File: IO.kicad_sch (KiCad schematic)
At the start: 0 parts

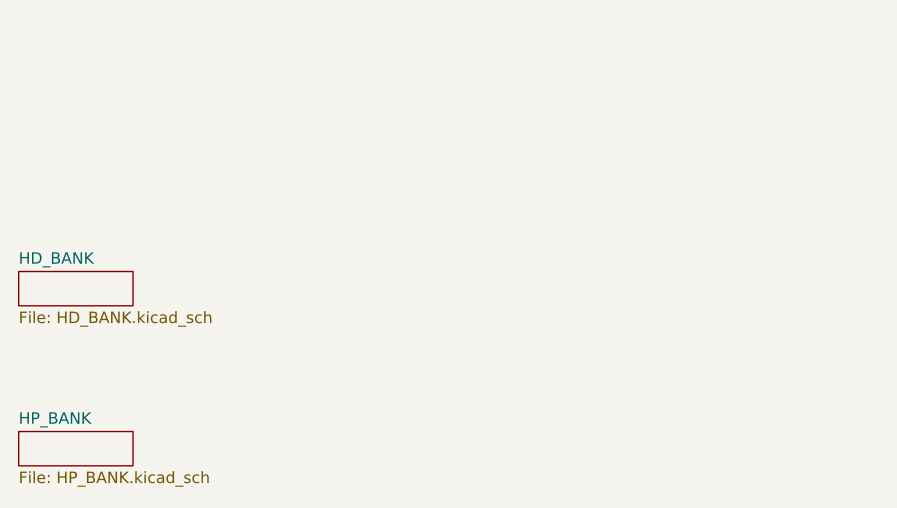
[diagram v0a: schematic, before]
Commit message: finishing schematic
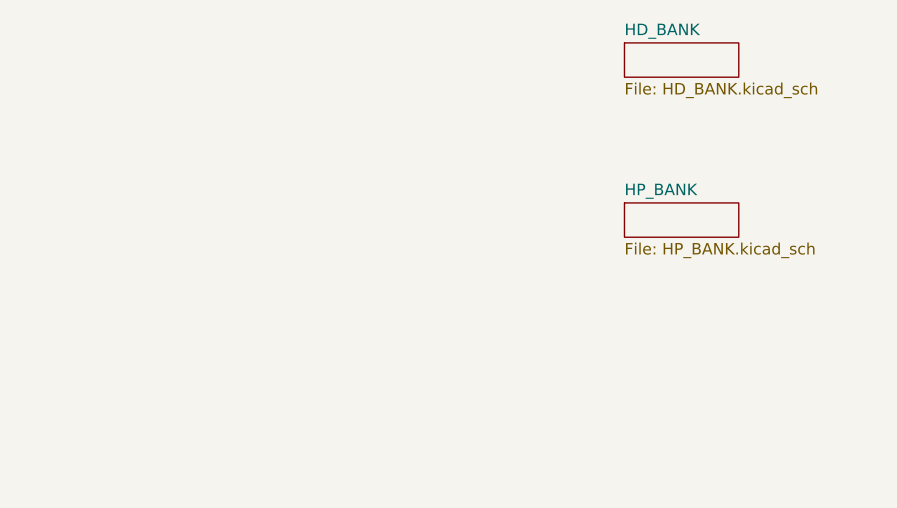
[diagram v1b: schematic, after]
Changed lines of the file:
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@@
 	(paper "A4")
 	(sheet
-		(at 74.93 121.92)
+		(at 142.24 96.52)
 		(size 12.7 3.81)
 		(exclude_from_sim no)
@@
 		)
 		(property "Sheetname" "HP_BANK"
-			(at 74.93 121.2084 0)
+			(at 142.24 95.8084 0)
 			(show_name no)
 			(do_not_autoplace no)
@@
 		)
 		(property "Sheetfile" "HP_BANK.kicad_sch"
-			(at 74.93 126.3146 0)
+			(at 142.24 100.9146 0)
 			(show_name no)
 			(do_not_autoplace no)
@@
 	)
 	(sheet
-		(at 74.93 104.14)
+		(at 142.24 78.74)
 		(size 12.7 3.81)
 		(exclude_from_sim no)
@@
 		)
 		(property "Sheetname" "HD_BANK"
-			(at 74.93 103.4284 0)
+			(at 142.24 78.0284 0)
 			(show_name no)
 			(do_not_autoplace no)
@@
 		)
 		(property "Sheetfile" "HD_BANK.kicad_sch"
-			(at 74.93 108.5346 0)
+			(at 142.24 83.1346 0)
 			(show_name no)
 			(do_not_autoplace no)
